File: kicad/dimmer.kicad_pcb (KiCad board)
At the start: 2 copper layers, 12 parts, among them IC1 ATTINY85-P, P1 CONN_01X02, P2 CONN_01X02, Q1 Q_NMOS_GDS, SW1 TACTILE_SW, SW2 TACTILE_SW, SW3 TACTILE_SW, SW4 TACTILE_SW, U1 MC78L05ACH

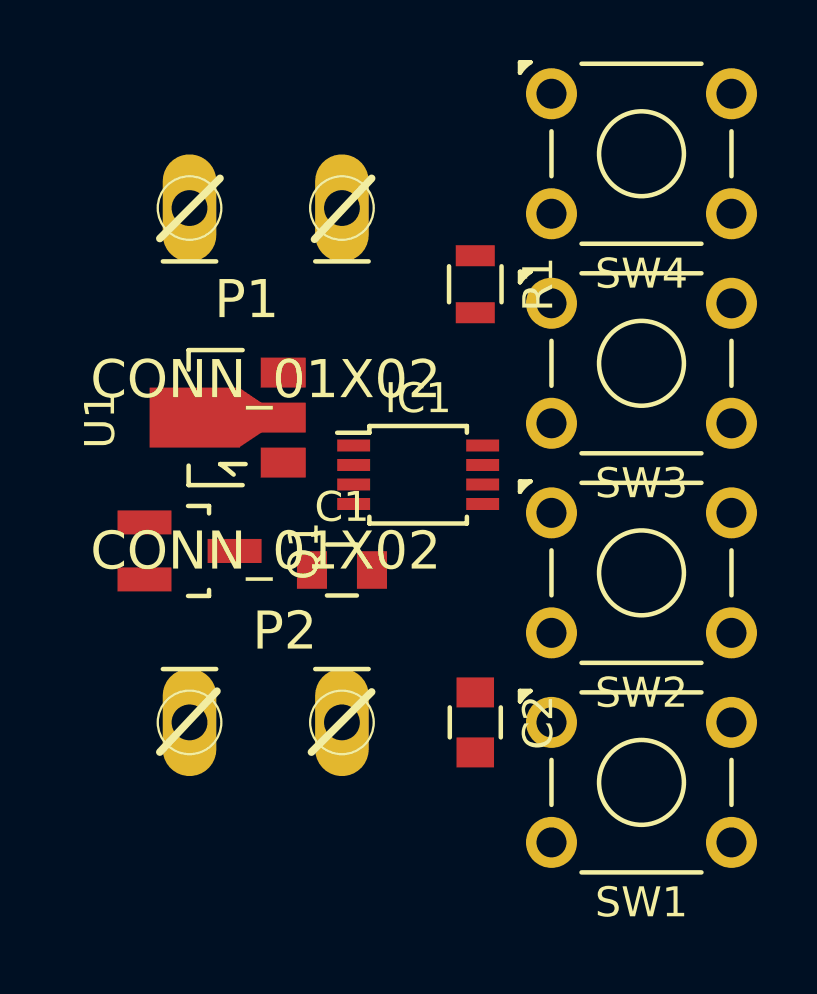
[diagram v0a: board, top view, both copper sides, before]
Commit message: pcb progress
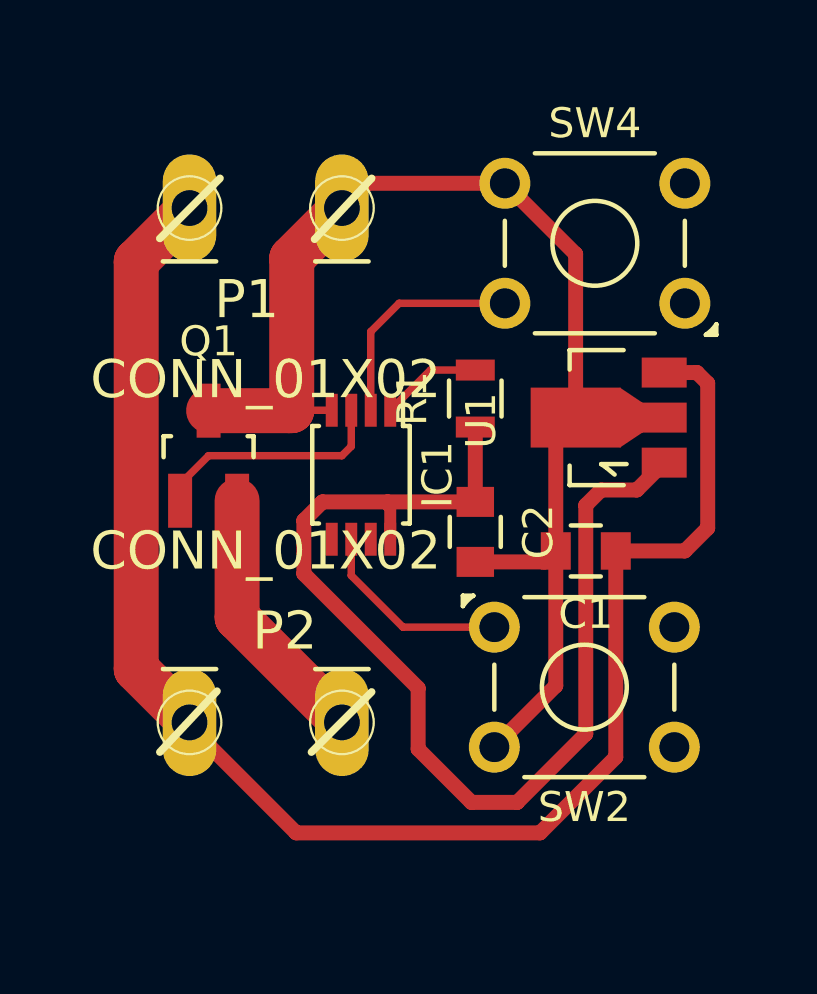
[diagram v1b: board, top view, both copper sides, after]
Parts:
- removed SW1, SW3: TACTILE_SW, Buttons_Switches_ThroughHole:SW_TH_Tactile_Omron_B3F-10xx
- moved U1 12.7 mm to (201.9, 127.6)
- moved SW4 8.28 mm to (204.5, 123.8), turned to 180 degrees
- moved C1 8.15 mm to (201.2, 132.1), turned to 180 degrees
- moved C2 6.35 mm to (197.5, 131.4)
- moved SW2 4.26 mm to (198.1, 134.6)
- moved R1 3.81 mm to (197.5, 127.0), turned to 90 degrees
- moved Q1 3.24 mm to (188.6, 128.9), turned to 0 degrees
- moved IC1 1.91 mm to (193.7, 129.5), turned to 270 degrees
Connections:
- IC1 pad 5: Net-(IC1-Pad5) -> (no net)
- IC1 pad 7: Net-(IC1-Pad7) -> (no net)
- P1 pad 1: GND -> +12V
- P1 pad 2: +12V -> GND
- SW4 pad 1: Net-(IC1-Pad2) -> (no net)
- SW4 pad 2: (no net) -> Net-(IC1-Pad2)
- SW4 pad 3: GND -> (no net)
- SW4 pad 4: (no net) -> GND
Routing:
- net +12V: track 0.00 -> 52.1 mm
- net GND: track 0.00 -> 41.5 mm
- net +5V: track 0.00 -> 37.3 mm
- net /out: track 0.00 -> 8.84 mm
- net Net-(IC1-Pad3): track 0.00 -> 7.98 mm
- net Net-(IC1-Pad2): track 0.00 -> 7.48 mm
- net Net-(IC1-Pad6): track 0.00 -> 6.77 mm
- net Net-(IC1-Pad1): track 0.00 -> 3.39 mm
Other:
- net class Load added: clearance 0.2, trace_width 1.5, via_dia 1.5, via_drill 0.8
- net class Power added: clearance 0.2, trace_width 0.5, via_dia 0.8, via_drill 0.6
